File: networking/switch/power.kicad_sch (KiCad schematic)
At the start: 8 parts, among them J1 DC IN, U1 AP2112K-3.3

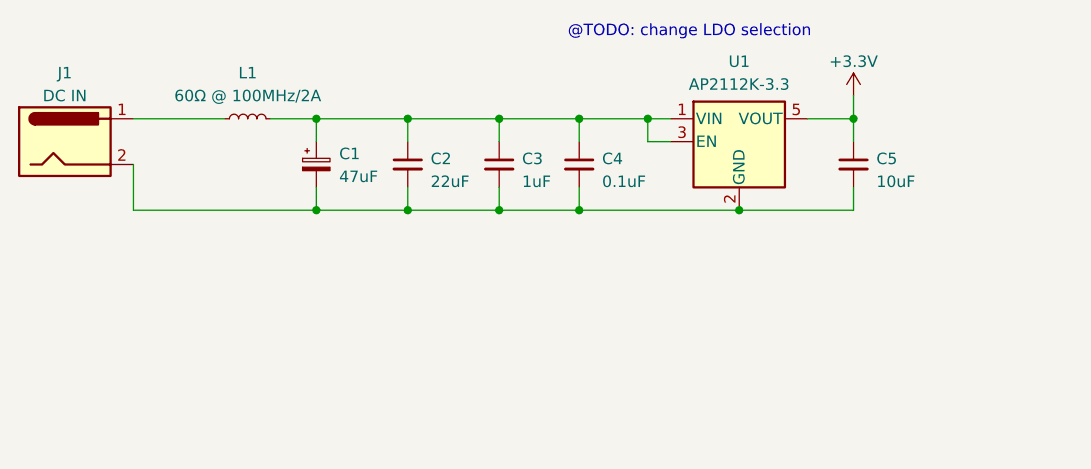
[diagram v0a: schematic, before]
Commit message: Feat[switch]: unpolished schematic complete
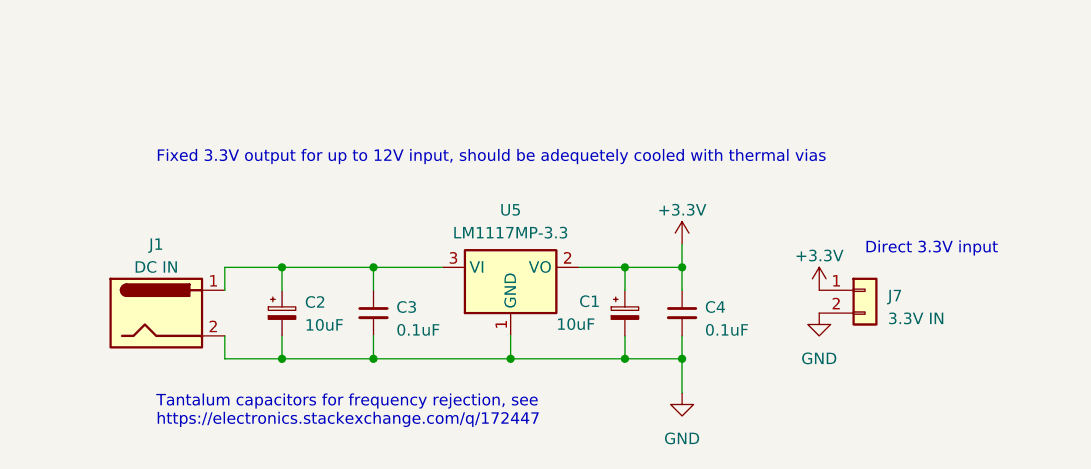
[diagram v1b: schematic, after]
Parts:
- removed C2: 22uF, symbol Device:C_Small
- removed C5: 10uF, symbol Device:C_Small
- removed L1: 60Ω @ 100MHz/2A, symbol Device:L_Small
- removed U1: AP2112K-3.3, Package_TO_SOT_SMD:SOT-23-5, symbol Regulator_Linear:AP2112K-3.3
- added C2: 10uF, symbol Device:C_Polarized_Small
- added J7: 3.3V IN, symbol Connector_Generic:Conn_01x02
- added U5: LM1117MP-3.3, Package_TO_SOT_SMD:SOT-223-3_TabPin2, symbol Regulator_Linear:LM1117MP-3.3
- C1: value 47uF -> 10uF
- C3: value 1uF -> 0.1uF
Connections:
- net +3.3V: now also C1.1, C4.1, J7.1 (Pin_1), U5.2 (VO)
- net at J1.1: now also C3.1, C2.1, U5.3 (VI)
- net GND: now reaches C1.2, C3.2, C4.2, J1.2
- net GND: now also C2.2, J7.2 (Pin_2), U5.1 (GND)
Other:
- note added: "Direct 3.3V input"
- note added: "Fixed 3.3V output for up to 12V input, should be adequetely cooled with thermal vias"
- note added: "Tantalum capacitors for frequency rejection, see https://electronics.stackexchange.com/q/172447"
- note removed: "@TODO: change LDO selection"
- moved on the sheet: J1
